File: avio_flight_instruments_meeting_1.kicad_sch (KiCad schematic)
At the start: 55 parts, among them J1 Conn_01x02_Male, J2 Conn_Coaxial, U1 MS5803-01BA_Miniature_Altimet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, U2 DS3231M, U3 RFM96W-433S2, U4 M20050-1, U5 BNO055

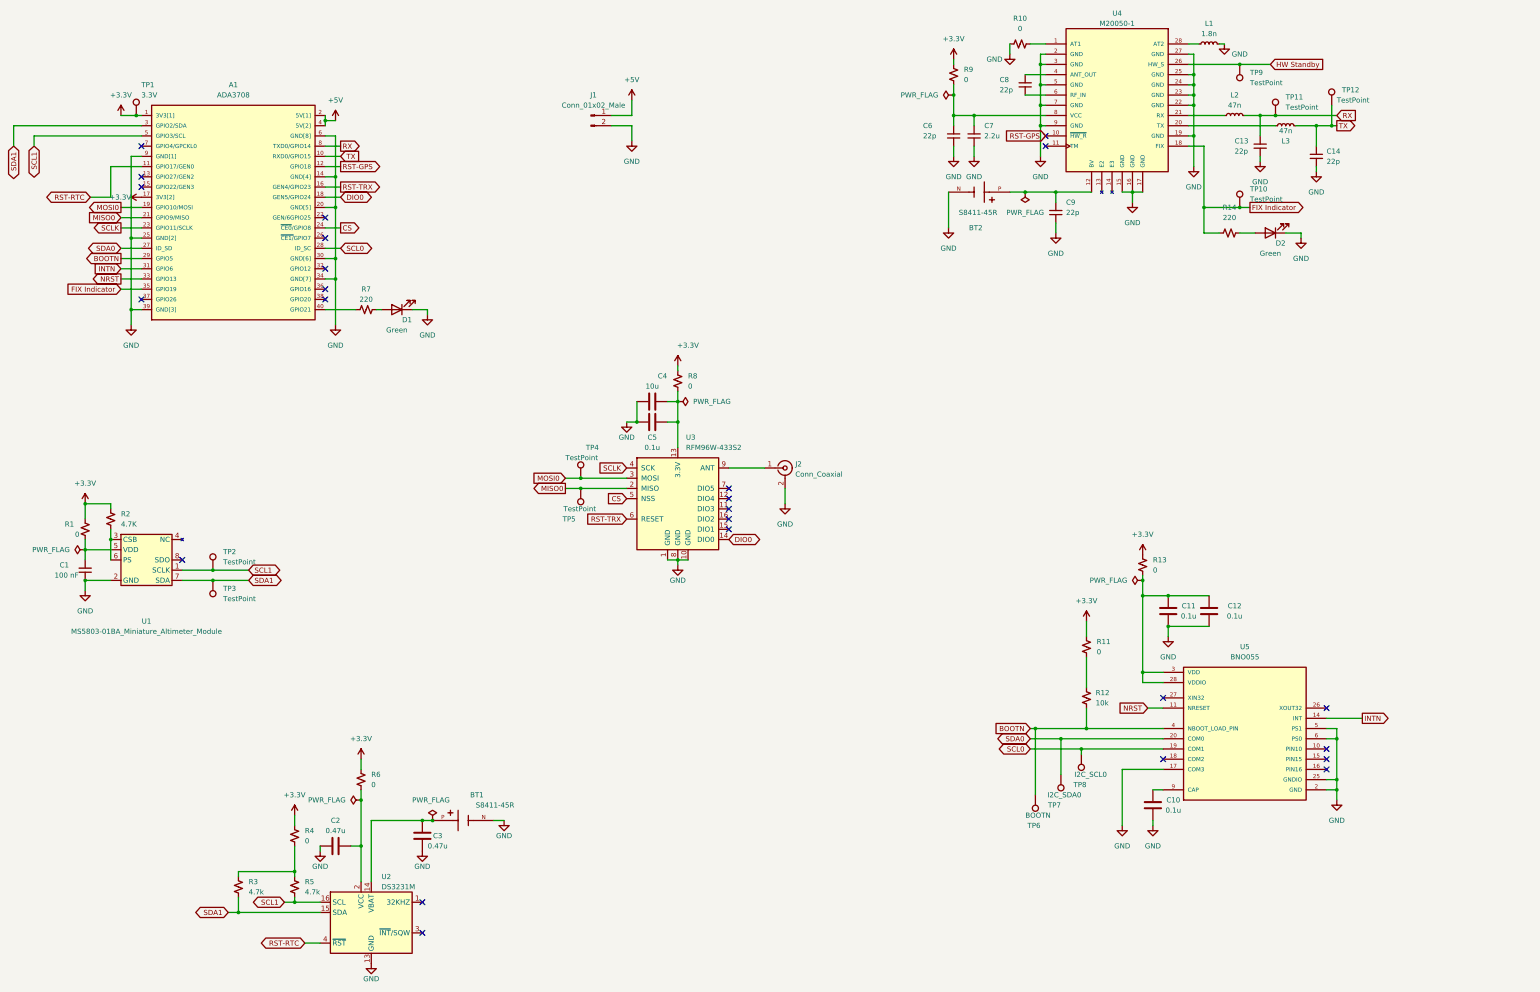
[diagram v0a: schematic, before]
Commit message: update 11_17
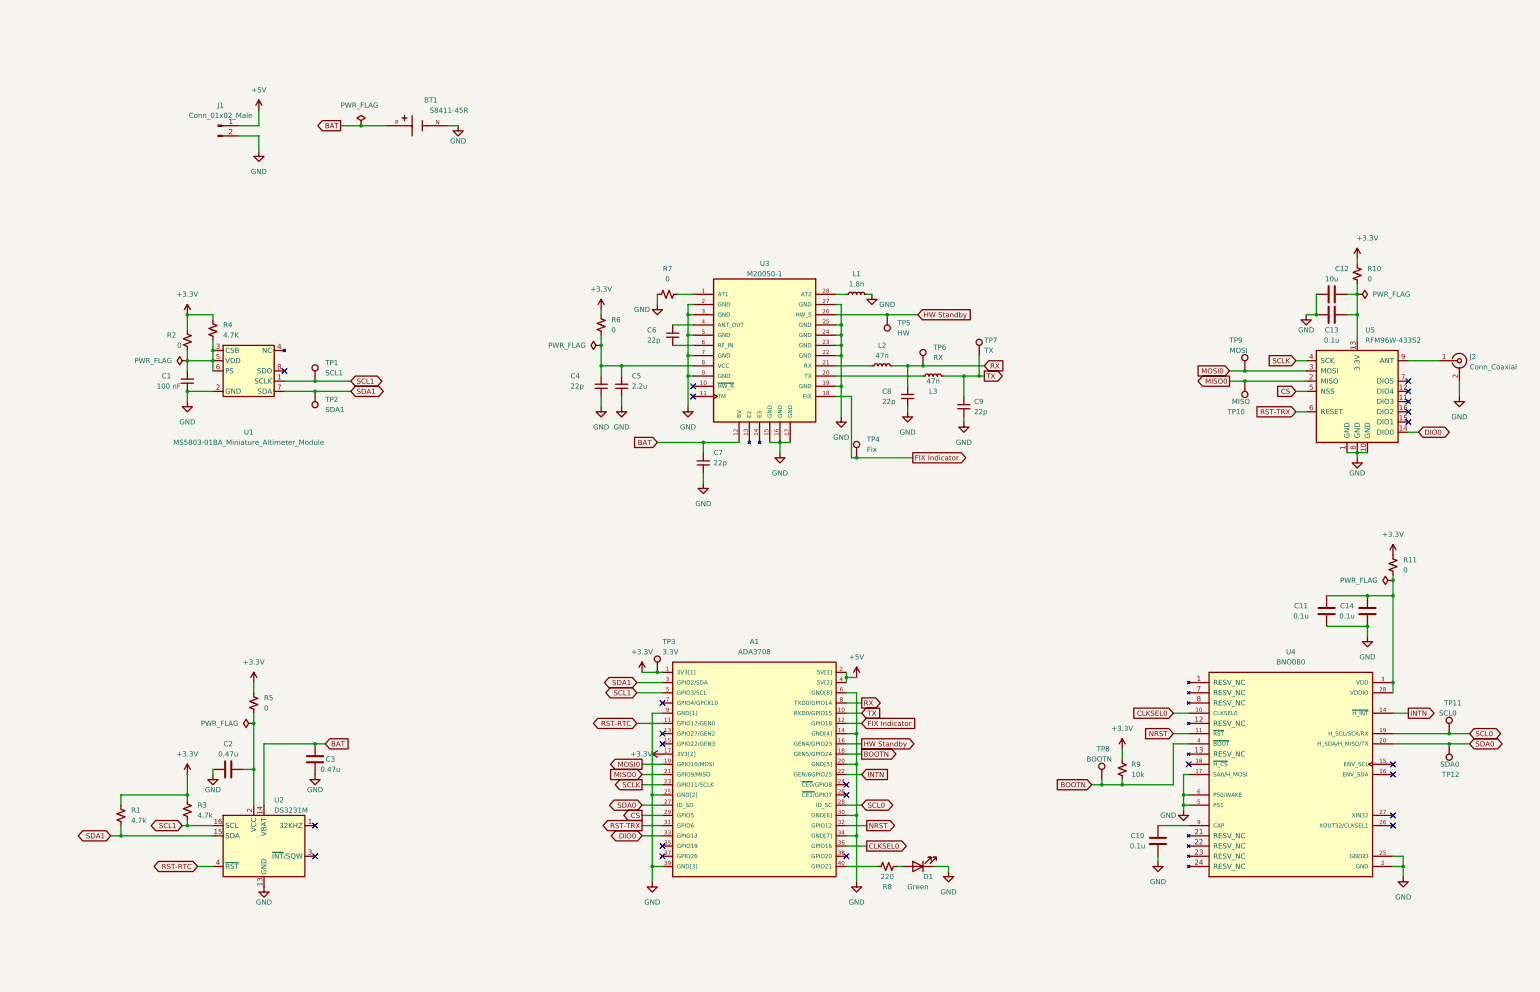
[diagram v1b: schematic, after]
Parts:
- removed BT2: S8411-45R, avio_flight_instruments_meeting_1:BAT_S8411-45R, symbol S8411-45R:S8411-45R
- removed D2: Green, LED_THT:LED_D3.0mm, symbol Device:LED
- removed R11, R4: 0, Resistor_SMD:R_1206_3216Metric, symbol Device:R_Small_US
- removed R14: 220, Resistor_SMD:R_1206_3216Metric, symbol Device:R_Small_US
- removed R3: 4.7k, Resistor_SMD:R_1206_3216Metric, symbol Device:R_Small_US
- removed TP6: BOOTN, TestPoint:TestPoint_Pad_D1.5mm, symbol Connector:TestPoint
- removed U5: BNO055, avio_flight_instruments_meeting_1:BNO085, symbol Flight_Instruments:BNO055
- added R1: 4.7k, Resistor_SMD:R_1206_3216Metric, symbol Device:R_Small_US
- added TP8: BOOTN, TestPoint:TestPoint_Pad_D1.5mm, symbol Connector:TestPoint
- added U4: BNO080, IC_BNO080, symbol Flight_Instruments:BNO080
- R4: renamed from R2; footprint (none) -> Resistor_SMD:R_1206_3216Metric
- TP1: renamed from TP2; value TestPoint -> SCL1
- TP10: renamed from TP5; value TestPoint -> MISO
- TP11: renamed from TP8; value I2C_SCL0 -> SCL0
- TP12: renamed from TP7; value I2C_SDA0 -> SDA0
- TP2: renamed from TP3; value TestPoint -> SDA1
- TP4: renamed from TP10; value TestPoint -> Fix
- TP5: renamed from TP9; value TestPoint -> HW
- TP6: renamed from TP11; value TestPoint -> RX
- TP7: renamed from TP12; value TestPoint -> TX
- TP9: renamed from TP4; value TestPoint -> MOSI
- renumbered C12 to C11, C4 to C12, C5 to C13, C11 to C14, C6 to C4, C7 to C5, C8 to C6, C9 to C7, C13 to C8, C14 to C9, R8 to R10, R13 to R11, R1 to R2, R5 to R3, R6 to R5, R9 to R6, R10 to R7, R7 to R8, R12 to R9, TP1 to TP3, U4 to U3, U3 to U5
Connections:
- net +3.3V: now also R3.1, R9.1, R1.1
- net BOOTN: now also A1.18 (GEN5/GPIO24), TP8.1, U4.4 (~{BOOT}); no longer A1.29 (GPIO5)
- net CS: now also A1.29 (GPIO5); no longer A1.24 (~{CE0}/GPIO8)
- net DIO0: now also A1.33 (GPIO13); no longer A1.18 (GEN5/GPIO24)
- net FIX Indicator: now also A1.12 (GPIO18); no longer A1.35 (GPIO19)
- net GND: now also U4.17 (SA0/H_MOSI), U4.2 (GND), U4.25 (GNDIO), U4.5 (PS1), U4.6 (PS0/WAKE)
- net HW Standby: now also A1.16 (GEN4/GPIO23)
- net INTN: now also A1.22 (GEN/6GPIO25), U4.14 (~{H_INT}); no longer A1.31 (GPIO6)
- net NRST: now also A1.32 (GPIO12), U4.11 (~{RST}); no longer A1.33 (GPIO13)
- net RST-TRX: now also A1.31 (GPIO6); no longer A1.16 (GEN4/GPIO23)
- net SCL0: now also U4.19 (H_SCL/SCK/RX)
- net SDA0: now also U4.20 (H_SDA/H_MISO/TX)
- net SDA1: now also R1.2
- net BAT: now reaches BT1.P, C3.1, U2.14 (VBAT)
- net BAT: now also C7.2, U3.12 (BV)
- net at C1.2, R2.2, U1.5 (VDD): now also R4.2, U1.3 (CSB), U1.6 (PS)
- net at C11.2, C14.2, R11.2: now also U4.28 (VDDIO), U4.3 (VDD)
- net CLKSEL0: now reaches A1.36 (GPIO16)
- net CLKSEL0: now also U4.10 (CLKSEL0)
- net at C10.2: now also U4.9 (CAP)
- net RST-GPS: no longer names the net of U3.10 (~{HW_R})
- net RST-GPS: no longer A1.12 (GPIO18)
- no-connect marks 25 -> 23
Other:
- moved on the sheet: A1, BT1, C1, C10, C11, C12, C13, C14, C2, C3, C4, C5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

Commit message: Added layout version 1 11_23_22
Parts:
- U4: footprint IC_BNO080 -> avio_flight_instruments_meeting_1:IC_BNO080
- renumbered C4 to C1, C2 to C11, C11 to C12, C3 to C13, C5 to C2, C6 to C3, C7 to C4, C12 to C5, C13 to C6, C8 to C7, C9 to C8, C1 to C9, R6 to R1, R5 to R10, R7 to R2, R10 to R3, R2 to R4, R4 to R5, R8 to R6, R9 to R7, R1 to R8, R3 to R9, TP9 to TP1, TP8 to TP10, TP10 to TP2, TP4 to TP3, TP5 to TP4, TP6 to TP5, TP7 to TP6, TP3 to TP7, TP1 to TP8, TP2 to TP9, U3 to U1, U5 to U2, U1 to U3, U2 to U5
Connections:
- net BOOTN: now also A1.22 (GEN/6GPIO25); no longer A1.18 (GEN5/GPIO24)
- net CLKSEL0: now also A1.32 (GPIO12); no longer A1.36 (GPIO16)
- net CS: now also A1.16 (GEN4/GPIO23); no longer A1.29 (GPIO5)
- net DIO0: now also A1.18 (GEN5/GPIO24); no longer A1.33 (GPIO13)
- net INTN: now also A1.38 (GPIO20); no longer A1.22 (GEN/6GPIO25)
- net NRST: now also A1.36 (GPIO16); no longer A1.32 (GPIO12)
- net RST-RTC: now also A1.7 (GPIO4/GPCKL0); no longer A1.11 (GPIO17/GEN0)
- net RST-TRX: now also A1.12 (GPIO18); no longer A1.31 (GPIO6)
- net HW: now reaches A1.13 (GPIO27/GEN2)
- net HW: now also TP4.1, U1.26 (HW_S)
- net FIX Indicator renamed FIX
- net FIX: now also A1.11 (GPIO17/GEN0); no longer A1.12 (GPIO18)
- removed net HW Standby: A1.16 (GEN4/GPIO23), TP4.1, U1.26 (HW_S)
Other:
- moved on the sheet: A1, BT1, C1, C10, C11, C12, C13, C14, C2, C3, C4, C5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
